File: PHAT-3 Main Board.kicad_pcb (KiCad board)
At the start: 2 copper layers, 18 parts, among them P1 Power Terminal Block, P2 Power Terminal Block, P3 Power Terminal Block, P4 Power Terminal Block, Q1 IRLZ44N, U1 AHT21, U10 Logic Level Converter, U2 ESP32-S3 Dual-core SX1262, U3 BME280, U4 GY-521 MPU-6050, U5 LM2596, U6 GT-7U, U7 SCD41, U8 uCAM-III, U9 SD Card Reader

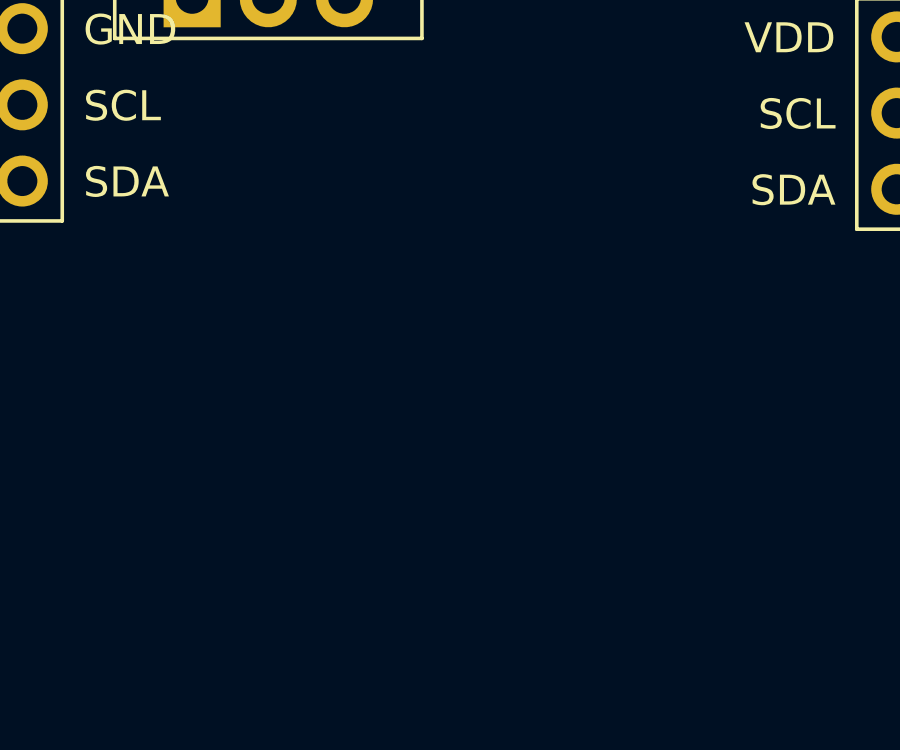
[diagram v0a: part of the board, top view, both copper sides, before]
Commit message: Rewired Everything Again
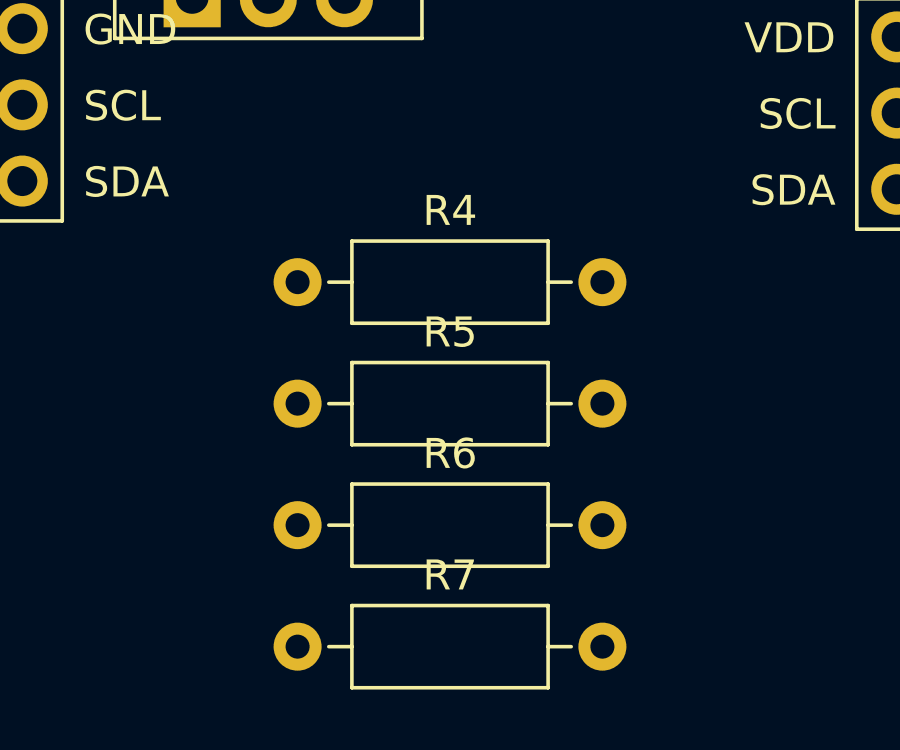
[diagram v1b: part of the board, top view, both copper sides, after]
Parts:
- added R4: 100, Resistor_THT:R_Axial_DIN0207_L6.3mm_D2.5mm_P10.16mm_Horizontal, F.Cu at (104.1, 142.8)
- added R5: 10k, Resistor_THT:R_Axial_DIN0207_L6.3mm_D2.5mm_P10.16mm_Horizontal, F.Cu at (104.1, 146.8)
- added R6: 10k, Resistor_THT:R_Axial_DIN0207_L6.3mm_D2.5mm_P10.16mm_Horizontal, F.Cu at (104.1, 150.9)
- added R7: 10k, Resistor_THT:R_Axial_DIN0207_L6.3mm_D2.5mm_P10.16mm_Horizontal, F.Cu at (104.1, 154.9)
- U3: value BME280 -> GY-68 BMP180; footprint Actual Footprint Library:BME280 -> Actual Footprint Library:GY-68 BMP180
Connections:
- R1 pad 2: Net-(U1-SDA) -> Net-(U10-HV1)
- R2 pad 1: Net-(U1-SCL) -> Net-(U10-HV2)
- U1 pad 1: +5V -> +3V3
- U10 pad 1: Net-(U10-LV1) -> Net-(U1-SCL)
- U10 pad 11: Net-(U1-SCL) -> Net-(U10-HV2)
- U10 pad 12: Net-(U1-SDA) -> Net-(U10-HV1)
- U10 pad 2: Net-(U10-LV2) -> Net-(U1-SDA)
- U10 pad 3: Net-(U10-LV) -> +3V3
- U2 pad 13: Net-(U10-LV2) -> Net-(U1-SCL)
- U2 pad 14: Net-(U10-LV1) -> Net-(U1-SDA)
- U2 pad 16: Net-(U10-LV) -> unconnected-(U2-3V3-Pad16)
- U2 pad 17: unconnected-(U2-3V3-Pad17) -> +3V3
- U2 pad 18: unconnected-(U2-GND-Pad18) -> GND
- U2 pad 28: Net-(Q1-G) -> Net-(U2-HTR)
- U3 pad 1: +5V -> +3V3
- U4 pad 3: Net-(U1-SCL) -> Net-(U10-HV1)
- U4 pad 4: Net-(U1-SDA) -> Net-(U10-HV2)
- U7 pad 1: unconnected-(U7-GND-Pad1) -> GND
- U7 pad 2: +5V -> +3V3
